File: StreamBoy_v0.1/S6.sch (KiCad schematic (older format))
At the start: 1 part, among them U1 XC6SLX9-TQG144

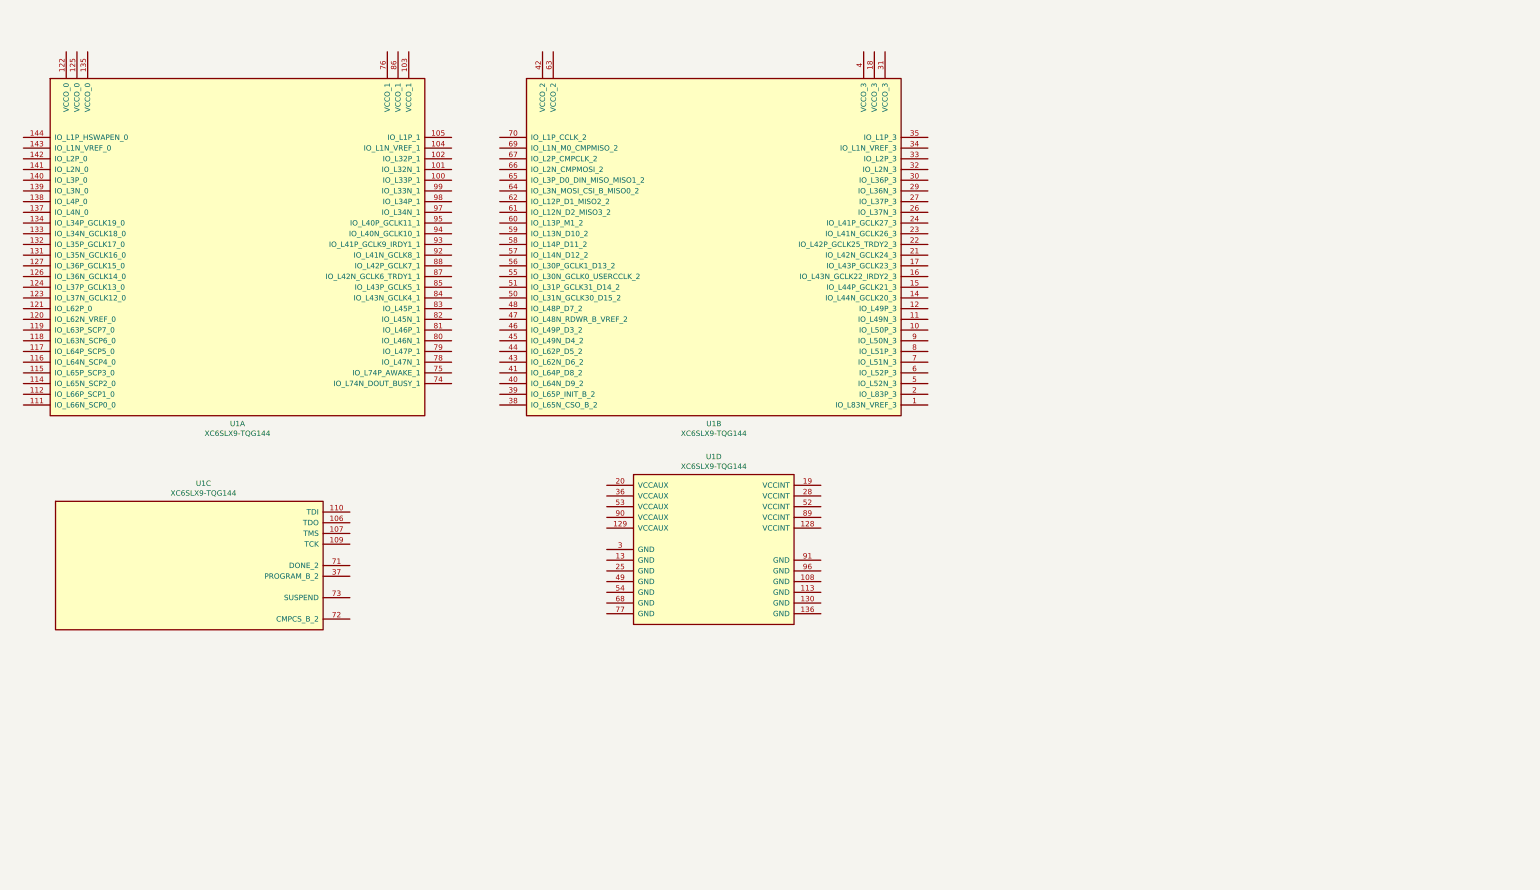
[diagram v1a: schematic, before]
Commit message: Bunch of stuff
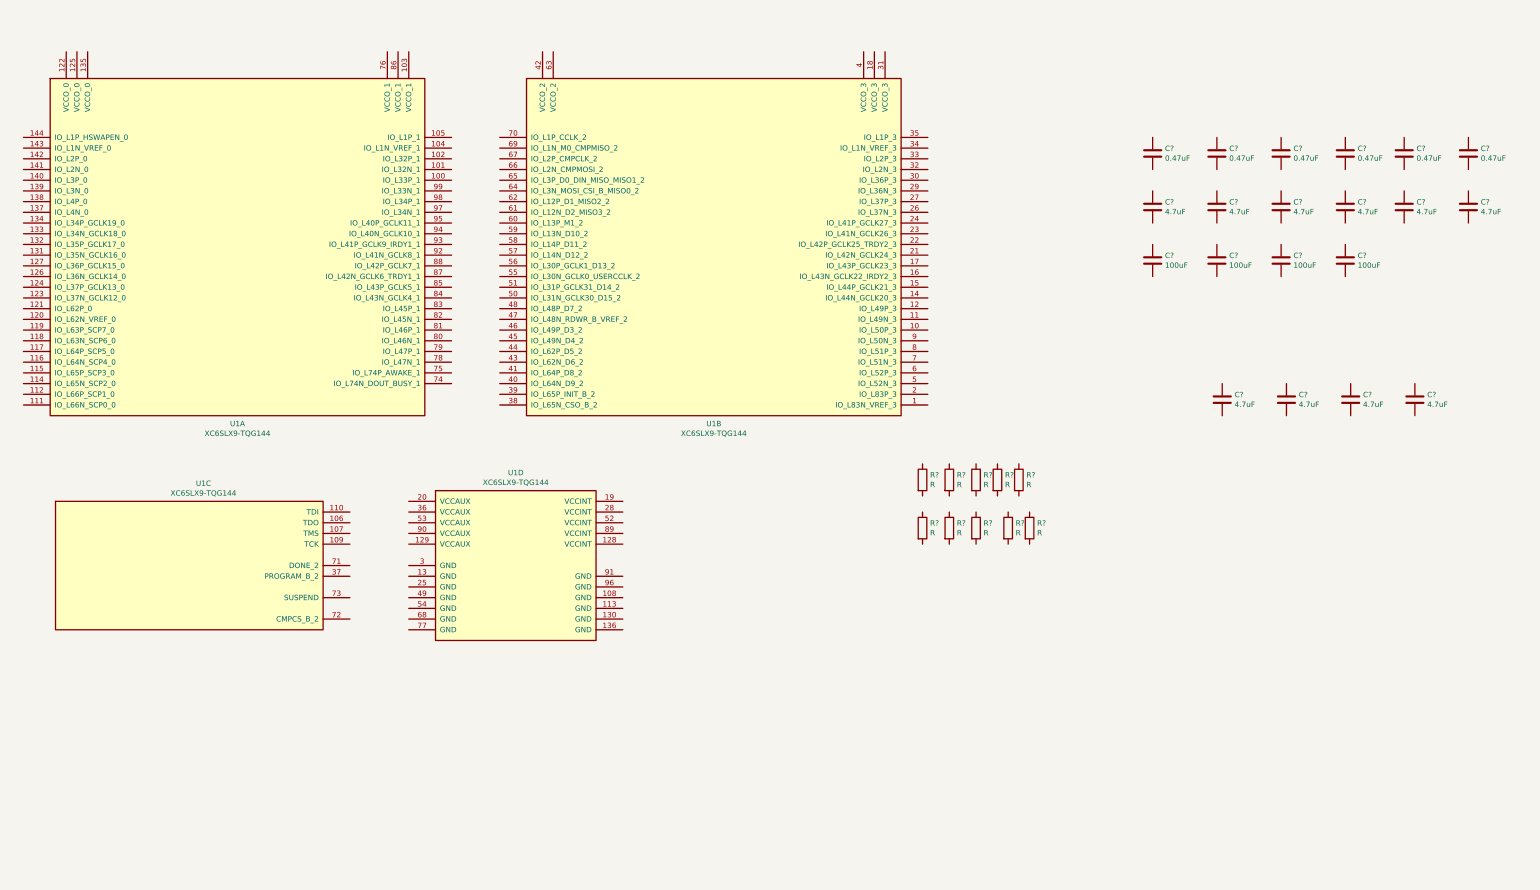
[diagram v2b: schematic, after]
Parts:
- added C? (x6): 0.47uF, Capacitor_SMD:C_0805_2012Metric, symbol Device:C
- added C? (x10): 4.7uF, Capacitor_SMD:C_0805_2012Metric, symbol Device:C
- added C? (x4): 100uF, Capacitor_SMD:C_0805_2012Metric, symbol Device:C
- added R? (x10): R, Resistor_SMD:R_0805_2012Metric, symbol Device:R
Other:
- moved on the sheet: U1D

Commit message: Power to the masses
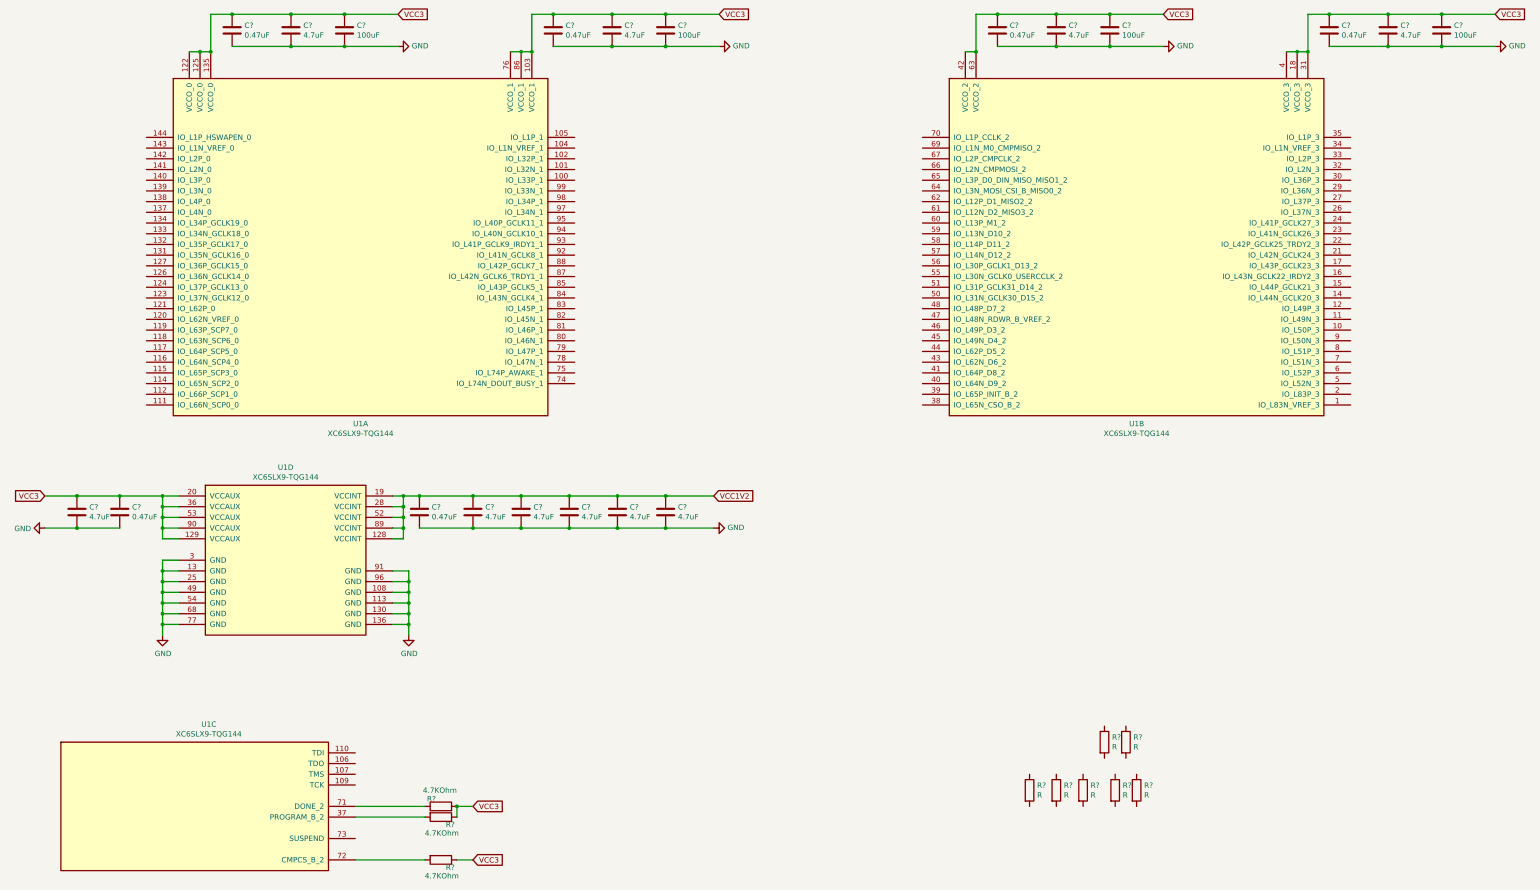
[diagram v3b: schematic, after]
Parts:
- removed C? (x3): 0.47uF, Capacitor_SMD:C_0805_2012Metric, symbol Device:C
- removed C? (x8): 4.7uF, Capacitor_SMD:C_0805_2012Metric, symbol Device:C
- removed C? (x3): 100uF, Capacitor_SMD:C_0805_2012Metric, symbol Device:C
- removed R? (x2): R, Resistor_SMD:R_0805_2012Metric, symbol Device:R
- added C? (x3): 0.47uF, Capacitor_SMD:C_0805_2012Metric, symbol Device:C
- added C? (x8): 4.7uF, Capacitor_SMD:C_0805_2012Metric, symbol Device:C
- added C? (x3): 100uF, Capacitor_SMD:C_0805_2012Metric, symbol Device:C
- added R? (x2): 4.7KOhm, Resistor_SMD:R_0805_2012Metric, symbol Device:R
- R?: value R -> 4.7KOhm
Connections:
- net VCC3: now reaches U1.103 (VCCO_1)
- net VCC3: now also C?.1, C?.1, C?.1, C?.1, C?.1, R?.2, U1.122 (VCCO_0), U1.125 (VCCO_0), U1.129 (VCCAUX), U1.135 (VCCO_0), U1.18 (VCCO_3), U1.20 (VCCAUX), U1.31 (VCCO_3), U1.36 (VCCAUX), U1.4 (VCCO_3), U1.42 (VCCO_2), U1.53 (VCCAUX), U1.63 (VCCO_2), U1.76 (VCCO_1), U1.86 (VCCO_1), U1.90 (VCCAUX), C?.1, C?.1, C?.1, C?.1, C?.1, C?.1, C?.1, C?.1, C?.1, R?.1, R?.1
- net GND: now reaches C?.2
- net GND: now also C?.2, C?.2, C?.2, C?.2, C?.2, U1.108 (GND), U1.113 (GND), U1.13 (GND), U1.130 (GND), U1.136 (GND), U1.25 (GND), U1.3 (GND), U1.49 (GND), U1.54 (GND), U1.68 (GND), U1.77 (GND), U1.91 (GND), U1.96 (GND), C?.2, C?.2, C?.2, C?.2, C?.2, C?.2, C?.2, C?.2, C?.2, C?.2, C?.2, C?.2, C?.2, C?.2
- net VCC1V2: now reaches C?.1
- net VCC1V2: now also U1.128 (VCCINT), U1.19 (VCCINT), U1.28 (VCCINT), U1.52 (VCCINT), U1.89 (VCCINT), C?.1, C?.1, C?.1, C?.1, C?.1
- net at R?.1: now also U1.71 (DONE_2)
- net at U1.37 (PROGRAM_B_2): now also R?.2
- net at U1.72 (CMPCS_B_2): now also R?.2
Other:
- moved on the sheet: C?, R?, U1A, U1B, U1C, U1D
